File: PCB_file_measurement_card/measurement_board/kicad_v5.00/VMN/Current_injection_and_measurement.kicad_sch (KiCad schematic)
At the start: 12 parts, among them J12 Conn_01x08_Female, J13 Conn_01x02_Female, J14 Conn_01x02_Female, J15 Conn_01x08_Female, K3 AQY212EH, K4 AQY212EH, K5 AQY212EH, K6 AQY212EH, U5 1115-Adress=0X48

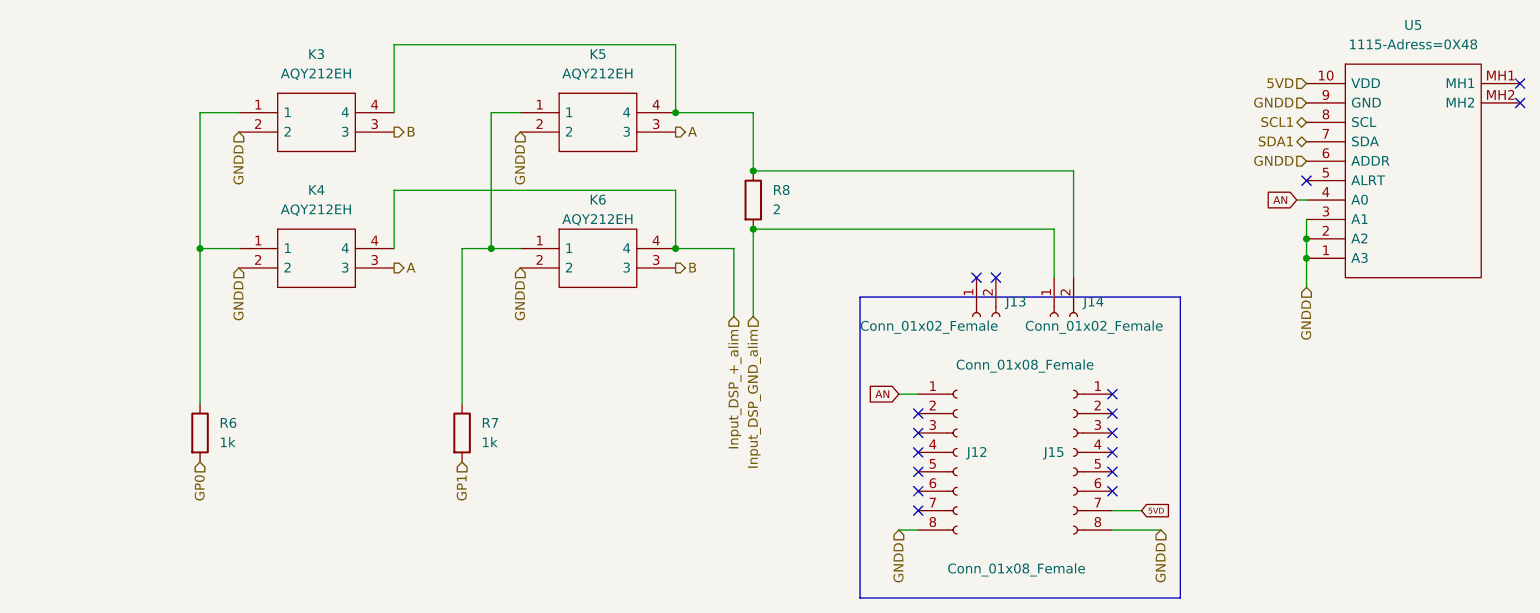
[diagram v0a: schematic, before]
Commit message: last version of measurement board, with op07
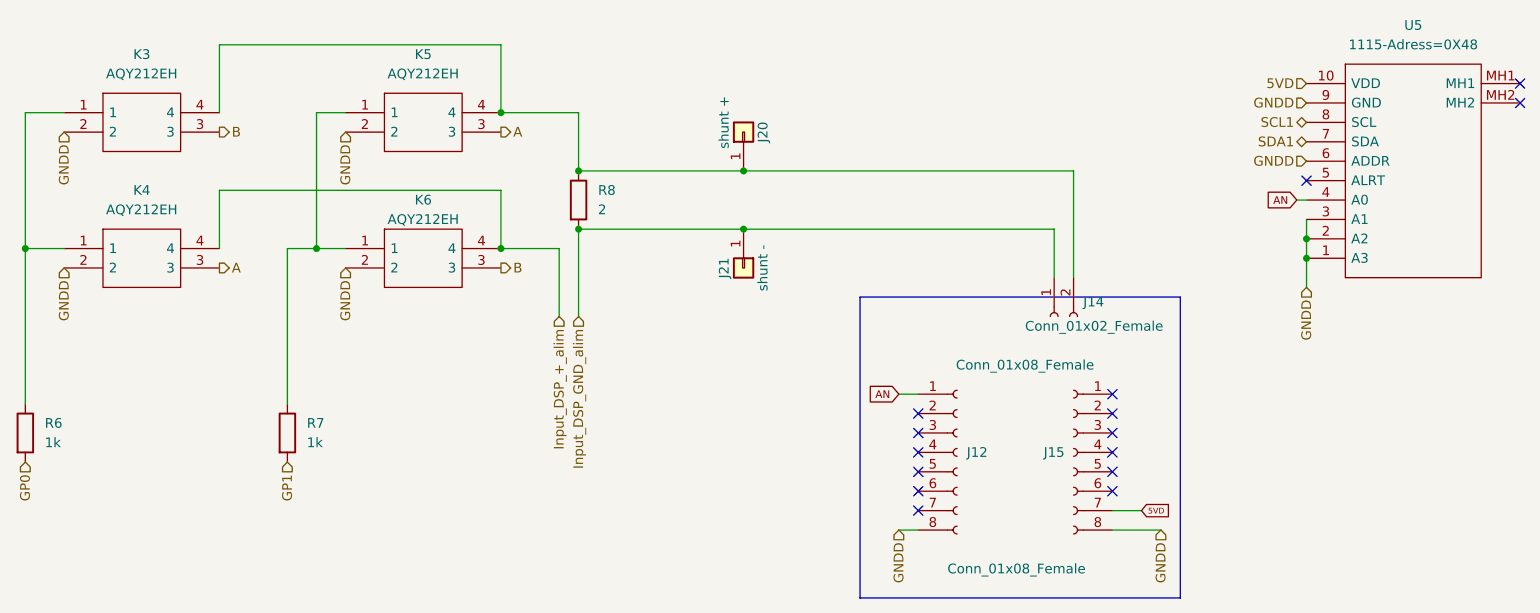
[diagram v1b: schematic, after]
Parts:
- removed J13: Conn_01x02_Female, Connector_PinHeader_2.54mm:PinHeader_1x02_P2.54mm_Vertical, symbol Connector:Conn_01x02_Female
- added J20: shunt +, Connector_PinHeader_2.54mm:PinHeader_1x01_P2.54mm_Vertical, symbol Connector_Generic:Conn_01x01
- added J21: shunt -, Connector_PinHeader_2.54mm:PinHeader_1x01_P2.54mm_Vertical, symbol Connector_Generic:Conn_01x01
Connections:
- net Input_DSP_GND_alim: now also J21.1 (Pin_1)
- net at J14.2 (Pin_2), K3.4, K5.4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: now also J20.1 (Pin_1)
- no-connect marks 17 -> 15
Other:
- moved on the sheet: K3, K4, K5, K6, R6, R7, R8
